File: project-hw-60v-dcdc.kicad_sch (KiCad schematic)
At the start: 0 parts

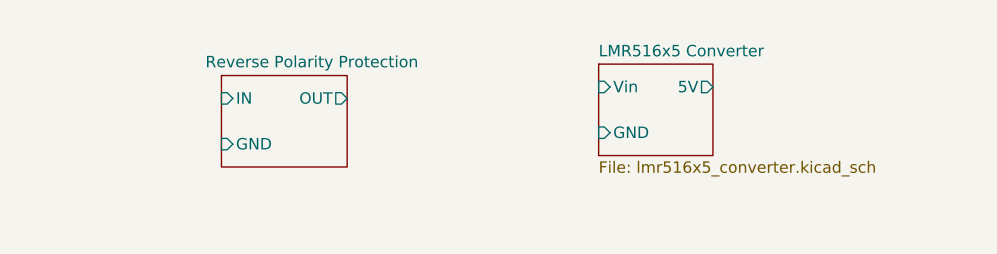
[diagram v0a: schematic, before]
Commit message: sch: first draft
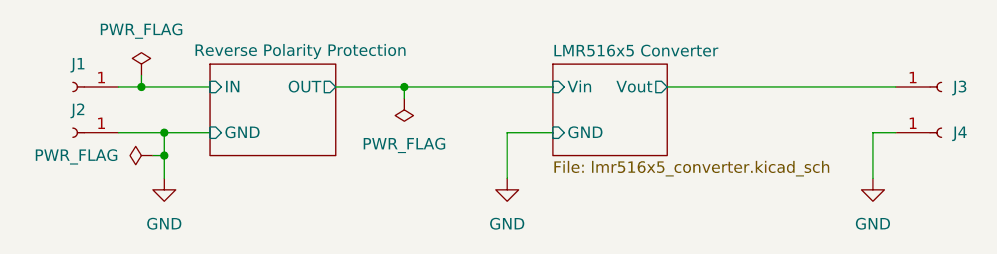
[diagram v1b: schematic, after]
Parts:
- added J1, J2, J3, J4: Conn_01x01_Socket, Connector_SolderPad:EdgePad_1x1, symbol Connector:Conn_01x01_Socket
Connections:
- net Reverse Polarity Protection/IN: now also J1.1 (Pin_1)
- new net GND: J2.1 (Pin_1), J4.1 (Pin_1)
- new net LMR516x5 Converter/Vout: J3.1 (Pin_1)
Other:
- sheet LMR516x5 Converter ports: added Vout; removed 5V
